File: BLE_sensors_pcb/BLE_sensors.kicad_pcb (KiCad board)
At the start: 2 copper layers, 49 parts, among them J1 Conn_ARM_SWD_TagConnect_TC203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, J2 Conn_01x02, J3 USB_C_Receptacle, U1 BME280, U2 LSM303AHTR, U3 TPS63031DSK, U4 ME54BS01, U5 MCP73871, U6 TLV70018_SOT23-5, U7 MCP2221AxST

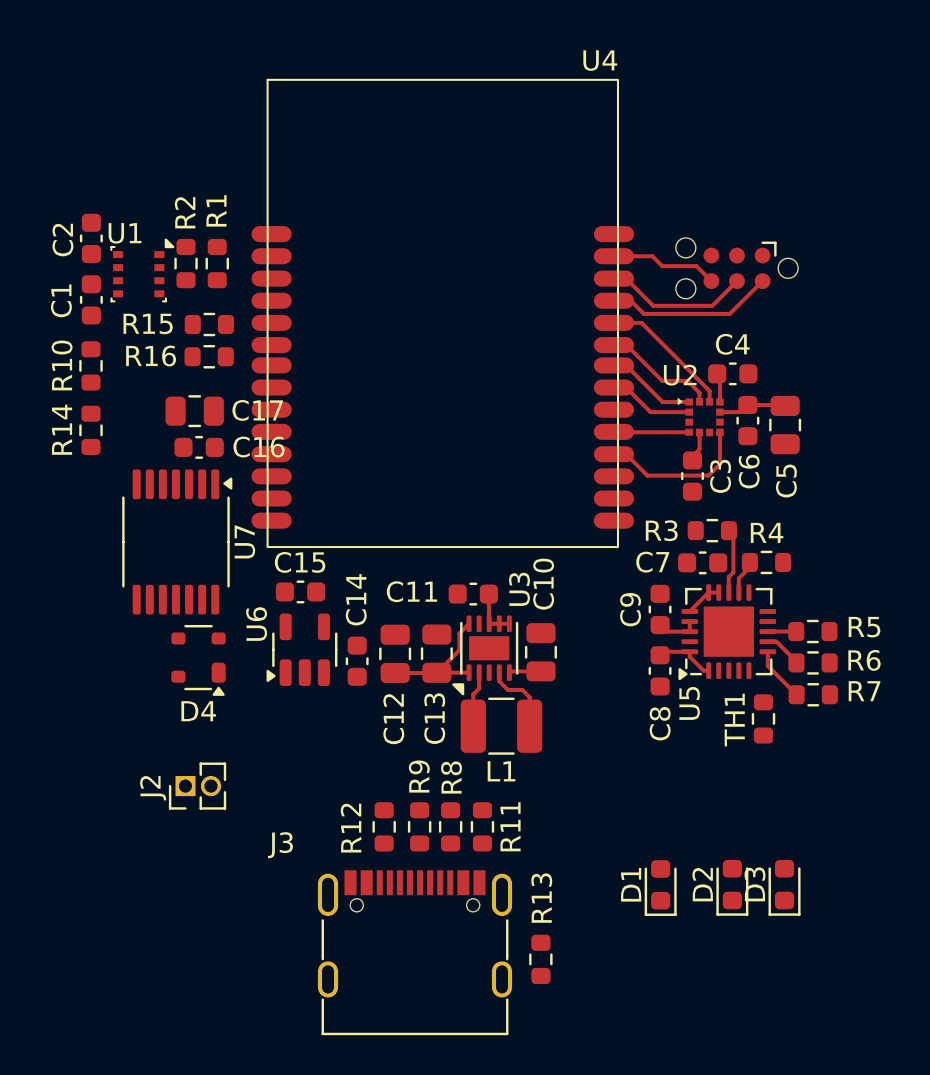
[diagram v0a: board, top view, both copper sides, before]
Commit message: save
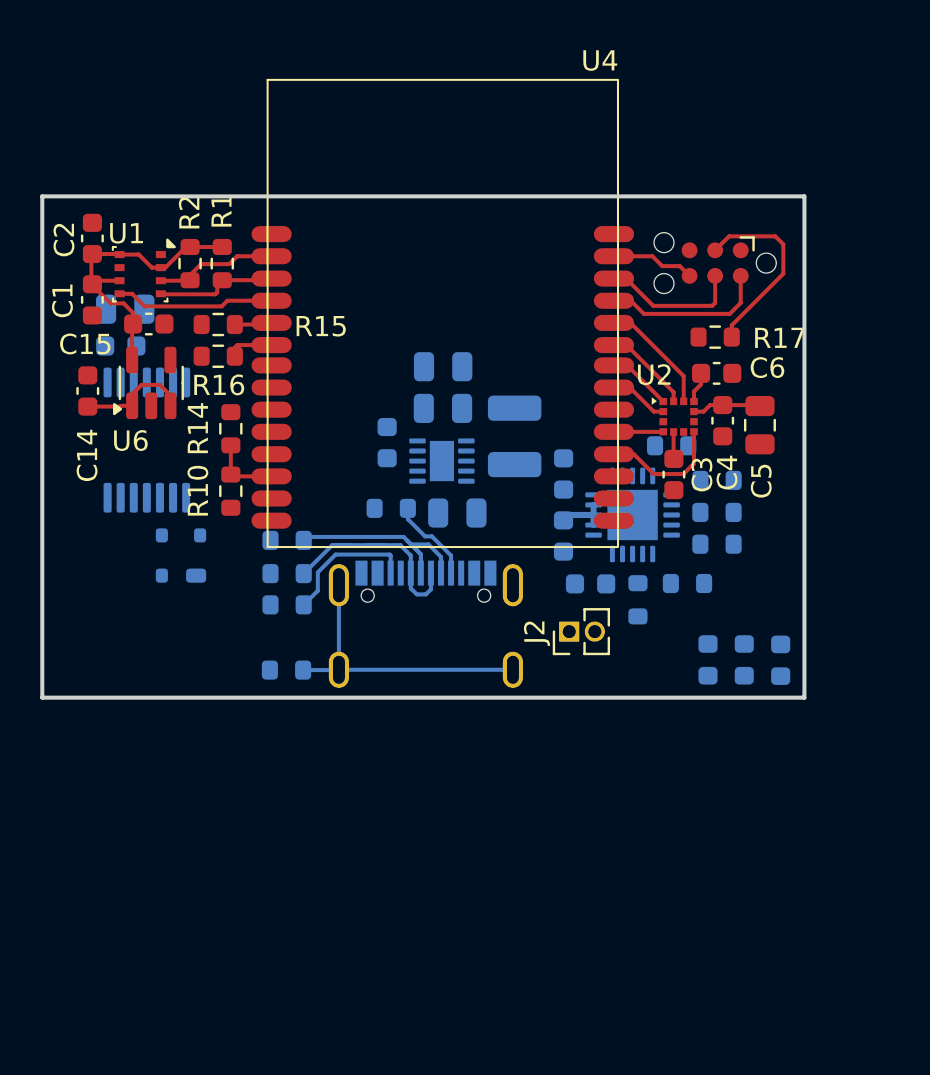
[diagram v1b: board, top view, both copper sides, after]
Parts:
- added R17: 10k, Resistor_SMD:R_0603_1608Metric, F.Cu at (154.8, 74.4)
- C10, C11, C12, C13, C16, C17, C7, C8, C9, D1, D2, D3, D4, J3, L1, R11, R12, R13, R3, R4, R5, R6, R7, R8, R9, TH1, U3, U5, U7: moved to B.Cu
- moved J2 20.5 mm to (147.6, 89.0)
- moved R13 19.1 mm to (133.5, 91.0), turned to 0 degrees
- moved C14 18.9 mm to (123.7, 77.1)
- moved R12 15.8 mm to (138.7, 82.9), turned to 0 degrees
- moved R9 15.7 mm to (133.6, 84.5), turned to 180 degrees
- moved J3 15.4 mm to (140.5, 89.9), turned to 180 degrees
- moved C15 15.3 mm to (126.7, 73.8)
- moved U6 15.3 mm to (126.8, 76.7)
- moved R8 15.0 mm to (133.6, 86.2), turned to 180 degrees
- moved R11 14.7 mm to (133.6, 87.7), turned to 0 degrees
- moved C12 14.5 mm to (141.3, 75.9), turned to 180 degrees
- moved L1 14.4 mm to (144.9, 79.4), turned to 90 degrees
- moved TH1 14.3 mm to (152.7, 79.8), turned to 0 degrees
- moved C13 12.2 mm to (141.3, 78.0), turned to 180 degrees
- moved R7 11.7 mm to (154.9, 81.5)
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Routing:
- net +1V8: track 0.00 -> 15.1 mm
- net Net-(J3-SHIELD): track 0.00 -> 14.6 mm
- net Net-(J3-D--PadA7): track 0.00 -> 10.4 mm
- net Net-(J3-D+-PadA6): track 0.00 -> 9.79 mm
- net /nRESET: track 0.00 -> 9.51 mm
- net /SDO: track 0.00 -> 7.92 mm
- net Net-(J3-CC2): track 0.00 -> 6.78 mm
- net /SDA: track 0.00 -> 6.15 mm
- net /SCL: track 0.00 -> 6.04 mm
- net /PWR_SUPPLY/Buck-Boost/Vin: track 4.62 -> 0.00 mm
- net Net-(J3-CC1): track 0.00 -> 4.30 mm
- net Net-(U3-L1): track 3.70 -> 0.00 mm
- net Net-(U4-P1.04/AIN0): track 0.00 -> 3.51 mm
- net Net-(U5-PROG1): track 3.26 -> 0.00 mm
- net Net-(U3-L2): track 2.78 -> 0.00 mm
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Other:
- board outline added: 37.8 x 24.9 mm
- copper layers 2 -> 4

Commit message: Added layers
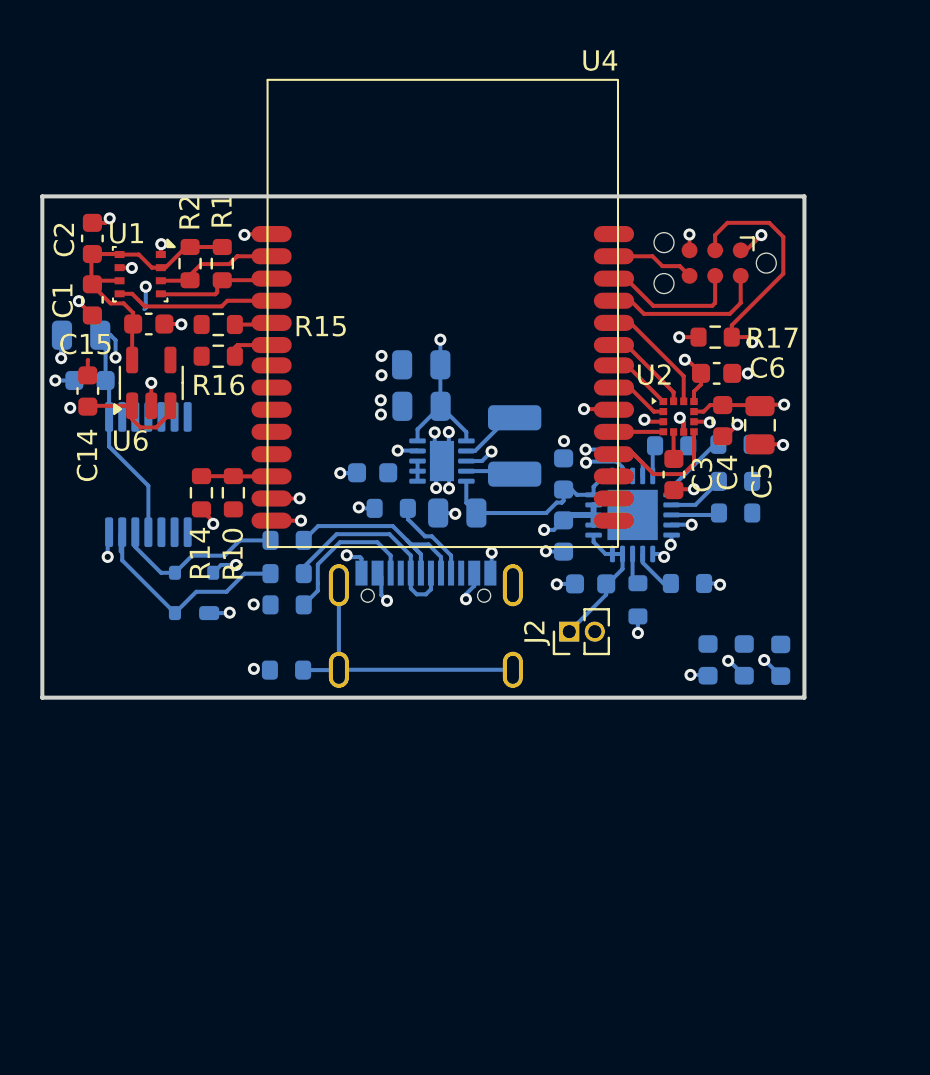
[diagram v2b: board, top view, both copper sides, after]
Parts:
- moved R14 3.50 mm to (129.3, 82.2), turned to -90 degrees
- moved C17 2.54 mm to (123.3, 74.3), turned to 180 degrees
- moved C13 2.42 mm to (140.2, 75.8)
- moved C16 2.30 mm to (123.8, 76.6), turned to 180 degrees
- moved C12 2.24 mm to (140.2, 77.9)
- moved R7 2.00 mm to (155.8, 79.8)
- moved D4 1.97 mm to (128.9, 87.1)
- moved R5 1.81 mm to (155.8, 83.2)
- moved R6 1.79 mm to (155.8, 81.6)
- moved U7 1.71 mm to (126.7, 81.2)
- moved C11 1.66 mm to (137.8, 81.2), turned to 180 degrees
- moved L1 0.48 mm to (144.9, 79.8)
- moved R10 0.15 mm to (130.9, 82.2)
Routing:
- net GND: track 0.00 -> 40.3 mm, vias 0 -> 46
- net +3V3: track 10.6 -> 39.9 mm, vias 0 -> 9
- net +5V: track 2.60 -> 17.1 mm, vias 0 -> 9
- net /nRESET: track 9.51 -> 23.1 mm, vias 0 -> 2
- net /usb-c/Protected_D+: track 0.00 -> 11.7 mm
- net /PWR_SUPPLY/Buck-Boost/Vin: track 0.00 -> 10.3 mm
- net /usb-c/Protected_D-: track 0.00 -> 8.65 mm
- net +V_bat: track 0.00 -> 7.02 mm
- net Net-(U5-~{PG}): track 0.00 -> 3.57 mm
- net Net-(U3-L2): track 0.00 -> 3.08 mm
- net Net-(U5-STAT2): track 0.00 -> 2.83 mm
- net Net-(U3-L1): track 0.00 -> 2.53 mm
- net Net-(U5-STAT1/~{LBO}): track 0.00 -> 2.39 mm
- net Net-(U5-PROG3): track 0.00 -> 2.26 mm
- net Net-(U5-PROG1): track 0.00 -> 1.56 mm
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- added copper zone on In2.Cu, net +3V3
- added copper zone on In2.Cu, net +5V
- added copper zone on In1.Cu, net GND
